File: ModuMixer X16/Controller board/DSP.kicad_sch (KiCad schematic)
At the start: 41 parts, among them Q3 MMBT2222A, Q4 MMBT2222A, U10 STM32F103RCTx, U11 4016, U6 LM358, U7 AMS1117-1.8, U8 LM324, U9 TLV320AIC3100

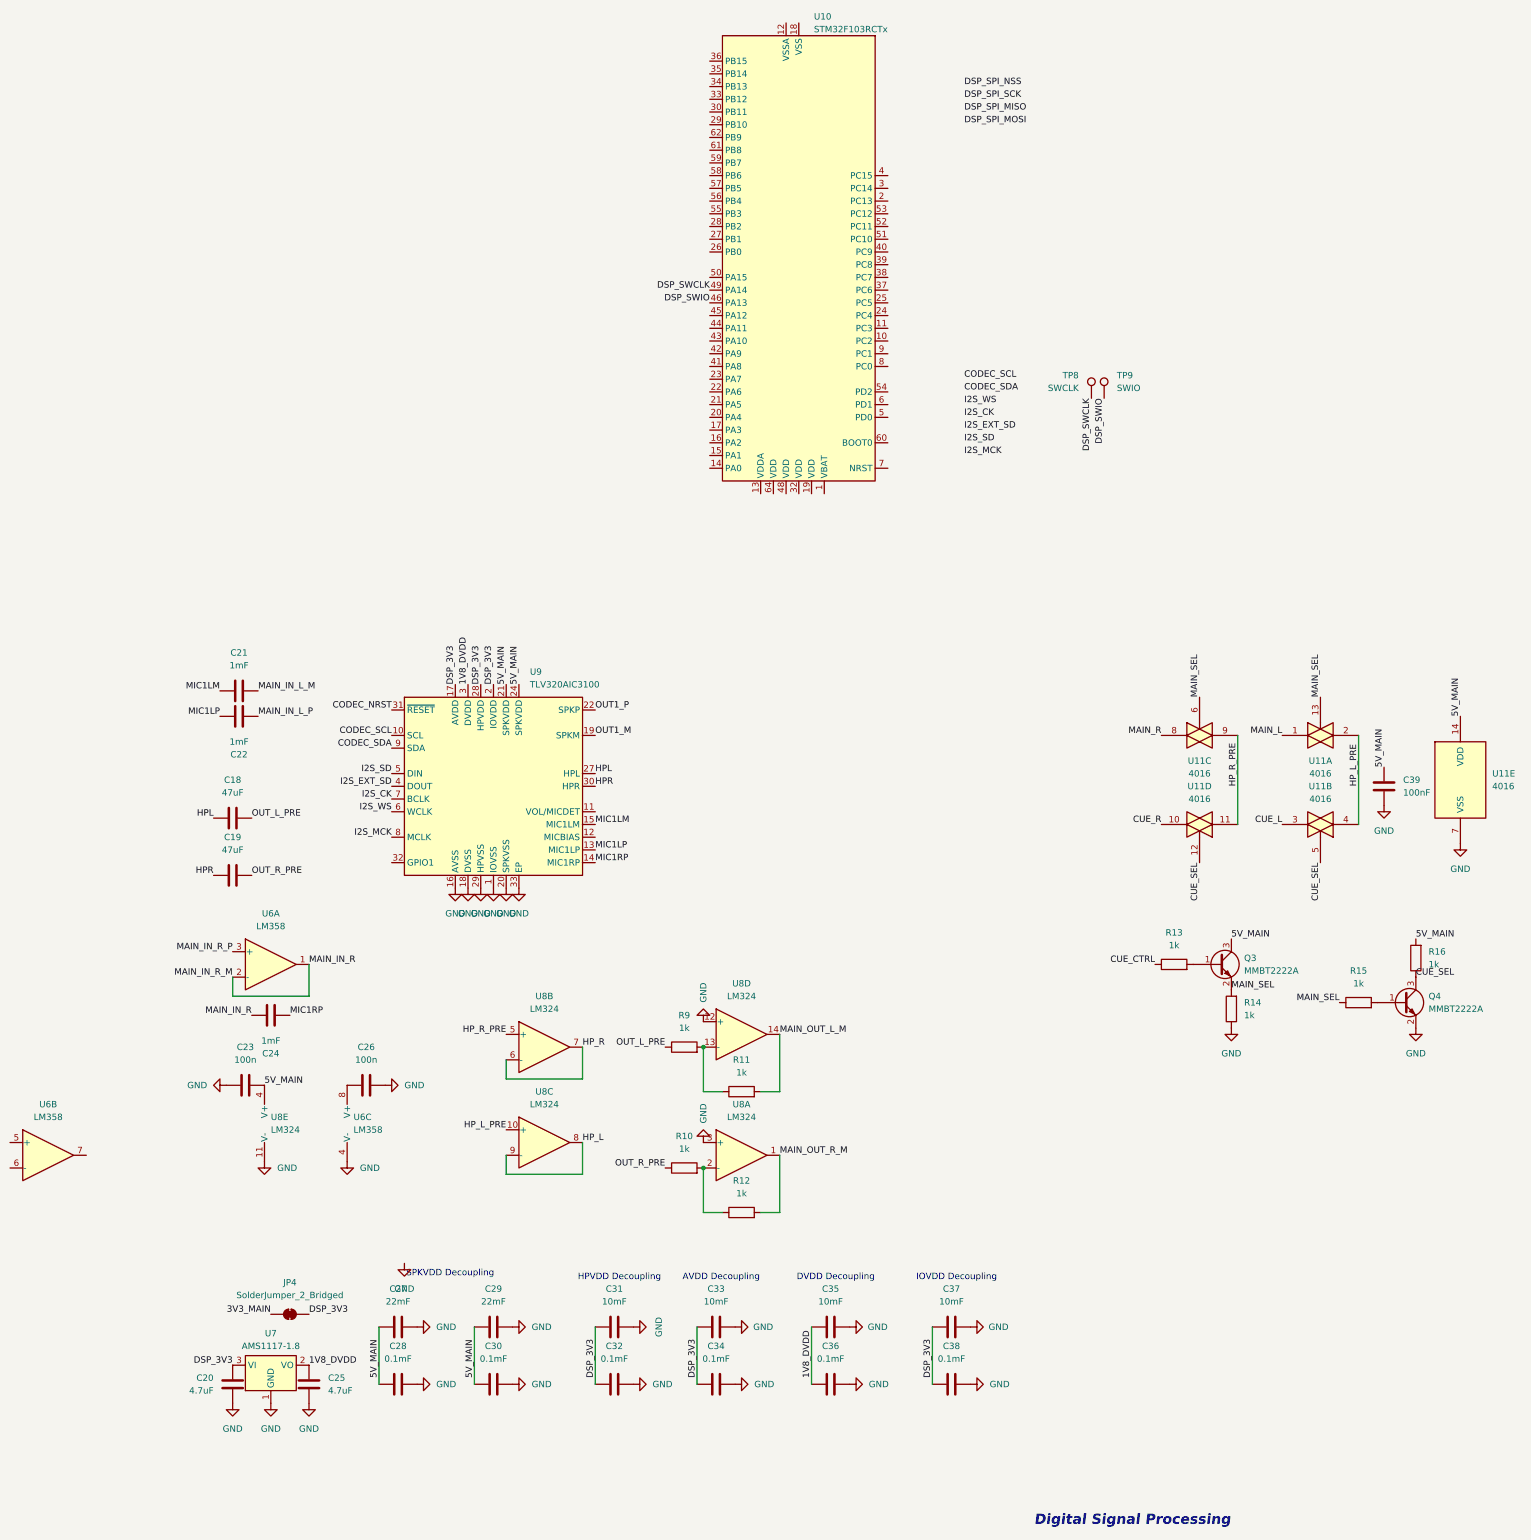
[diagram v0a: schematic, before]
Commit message: MCU replacement done
I finally did everything (i guess), i replaced the MCUs, set the clock components, connected them, idk i guess it's ok now, we just gotta make that pcb
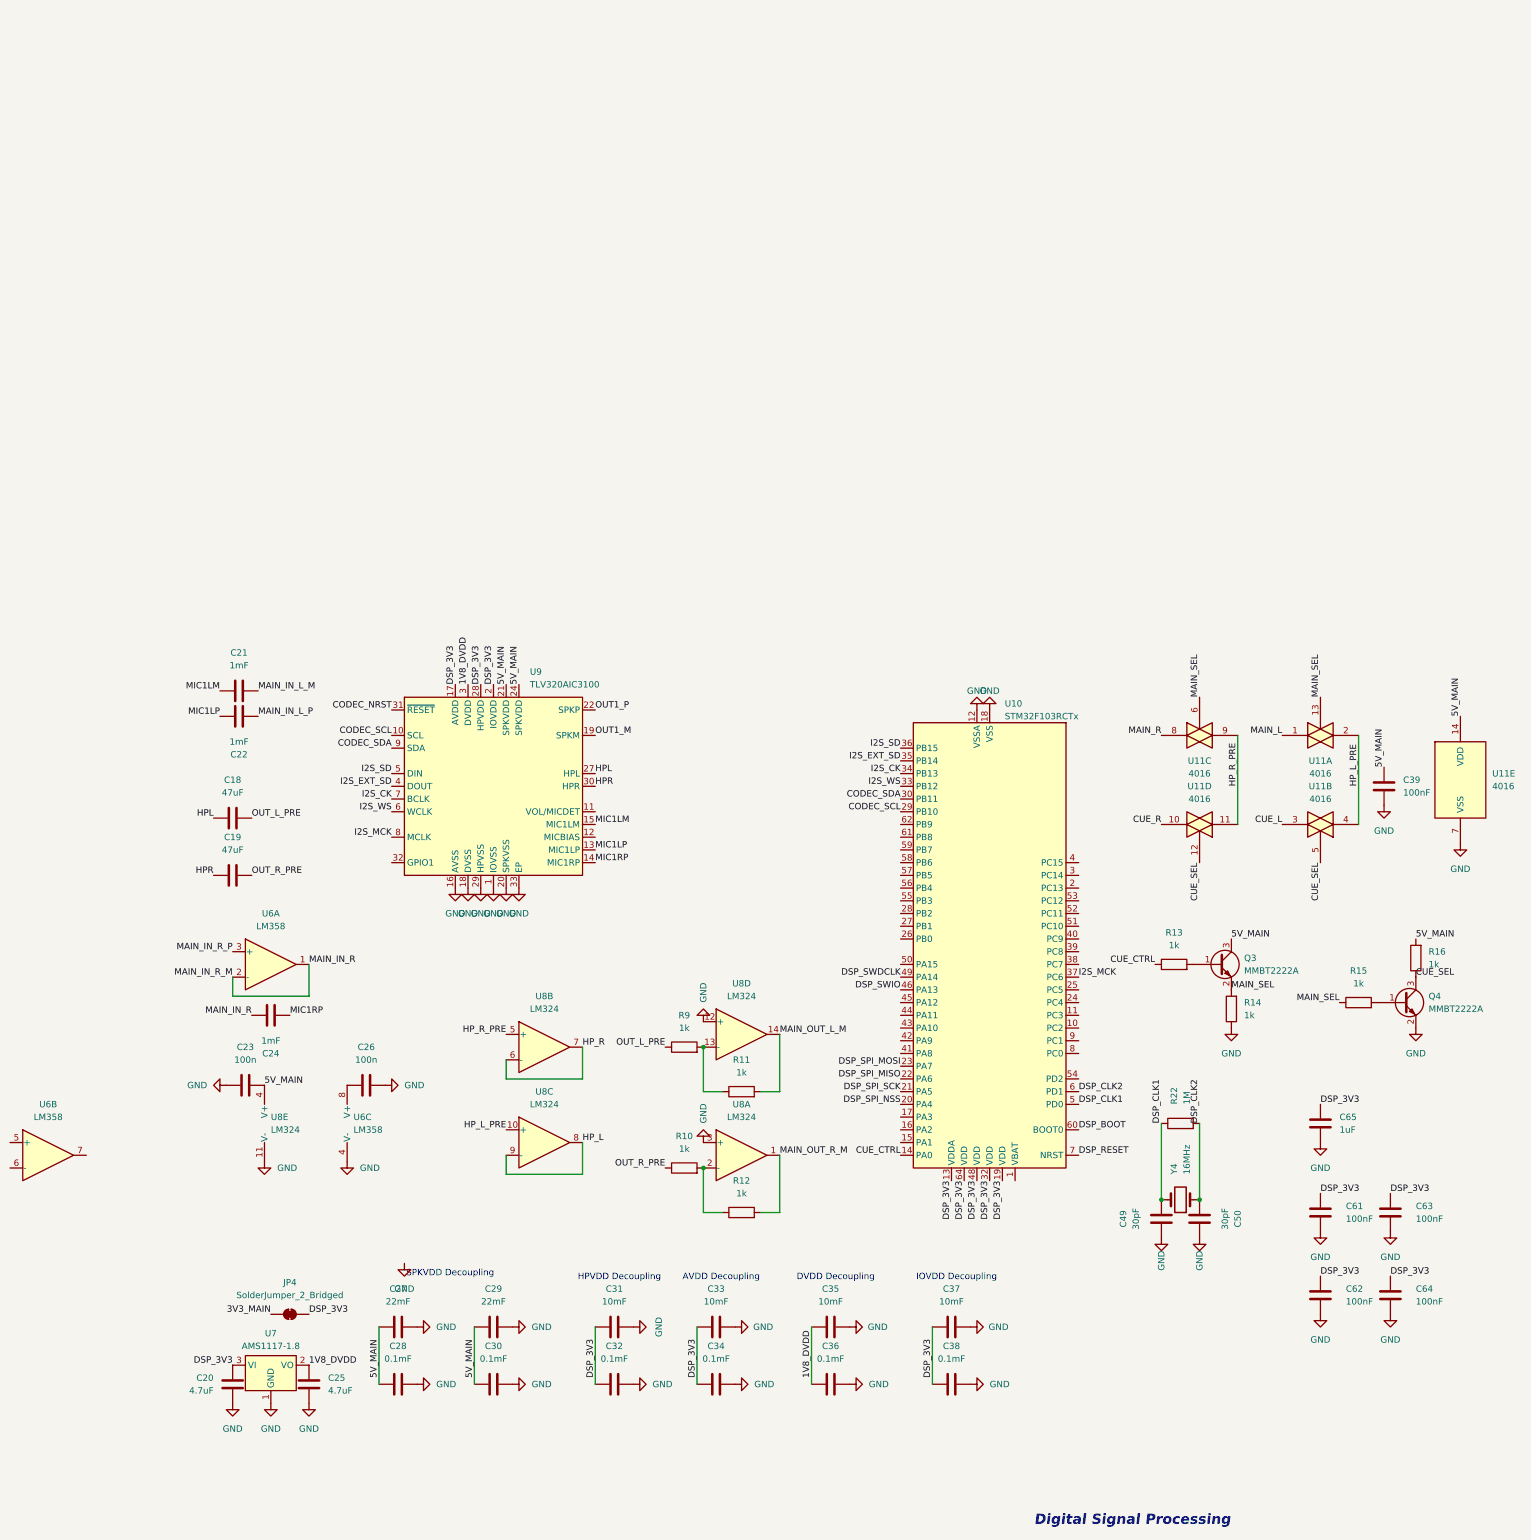
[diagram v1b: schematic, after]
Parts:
- removed TP8: SWCLK, TestPoint:TestPoint_Pad_D3.0mm, symbol Connector:TestPoint
- removed TP9: SWIO, TestPoint:TestPoint_Pad_D3.0mm, symbol Connector:TestPoint
- added C49, C50: 30pF, symbol Device:C
- added C61, C62, C63, C64: 100nF, symbol Device:C
- added C65: 1uF, symbol Device:C
- added R22: 1M, symbol Device:R
- added Y4: 16MHz, Crystal:Crystal_HC49-U_Vertical, symbol Device:Crystal
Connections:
- net CODEC_SCL: now also U10.29 (PB10)
- net CODEC_SDA: now also U10.30 (PB11)
- net CUE_CTRL: now also U10.14 (PA0)
- net DSP_3V3: now also U10.13 (VDDA), U10.19 (VDD), U10.32 (VDD), U10.48 (VDD), U10.64 (VDD), C61.1, C62.1, C63.1, C64.1, C65.1
- net DSP_SPI_MISO: now also U10.22 (PA6)
- net DSP_SPI_MOSI: now also U10.23 (PA7)
- net DSP_SPI_NSS: now also U10.20 (PA4)
- net DSP_SPI_SCK: now also U10.21 (PA5)
- net GND: now also U10.12 (VSSA), U10.18 (VSS), U10.31 (VSS), U10.47 (VSS), U10.63 (VSS), C49.2, C50.2, C61.2, C62.2, C63.2, C64.2, C65.2
- net I2S_CK: now also U10.34 (PB13)
- net I2S_EXT_SD: now also U10.35 (PB14)
- net I2S_MCK: now also U10.37 (PC6)
- net I2S_SD: now also U10.36 (PB15)
- net I2S_WS: now also U10.33 (PB12)
- net DSP_CLK1: now reaches U10.5 (PD0)
- net DSP_CLK1: now also C49.1, R22.1, Y4.2
- net DSP_CLK2: now reaches U10.6 (PD1)
- net DSP_CLK2: now also C50.1, R22.2, Y4.1
- net DSP_BOOT: now reaches U10.60 (BOOT0)
- net DSP_RESET: now reaches U10.7 (NRST)
- net DSP_SWCLK renamed DSP_SWDCLK
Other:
- moved on the sheet: U10
